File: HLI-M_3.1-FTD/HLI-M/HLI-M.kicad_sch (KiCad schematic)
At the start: 119 parts, among them CON1 , CON2 USB_B, CON3 , CON4 Con_ADAPTER, CON5 Con_MULTLINKER, CON6 Conn_01x15, CON7 Conn_01x09, CON8 CR123A, Q1 DMP3068L-7, Q2 BC817, Q3 BC817, Q4 DMP2305, Q5 DMP2305, Q6 DMP2305, Q7 DMP2305, U1 PIC24HJ64GP206, U10 ULN2003, U11 ULN2003, U12 ULN2003, U2 FM25V10, U3 MAX3232, U4 ATSHA204A-SSHDA-B, U5 24AA02-OT, U6 LM3658SD, U7 TPS7A0533PDBV, U8 TPS7A0533PDBV, U9 FT232RL, Y1 Crystal_32KHz, Y2 Crystal_20MHz

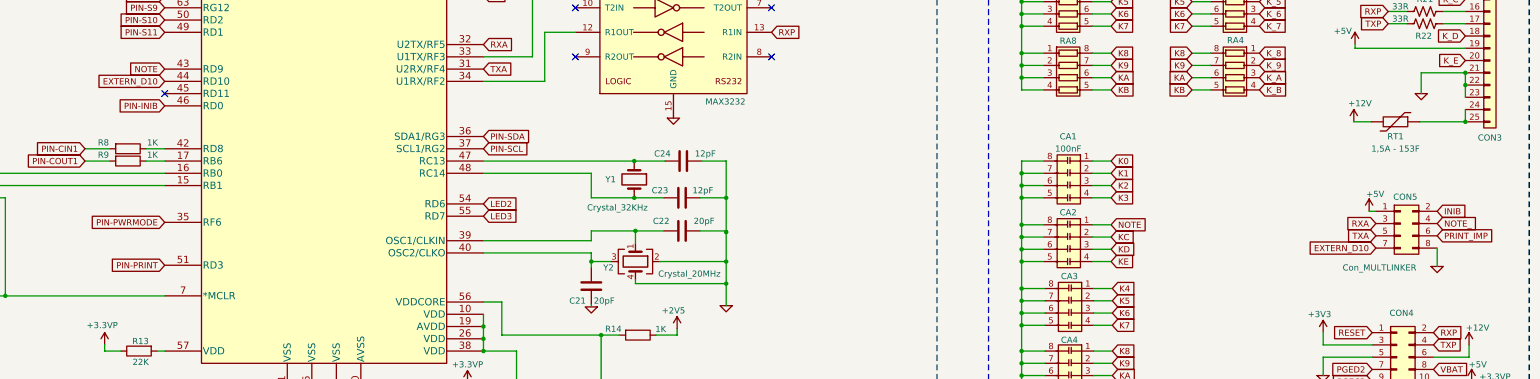
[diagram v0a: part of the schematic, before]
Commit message: att
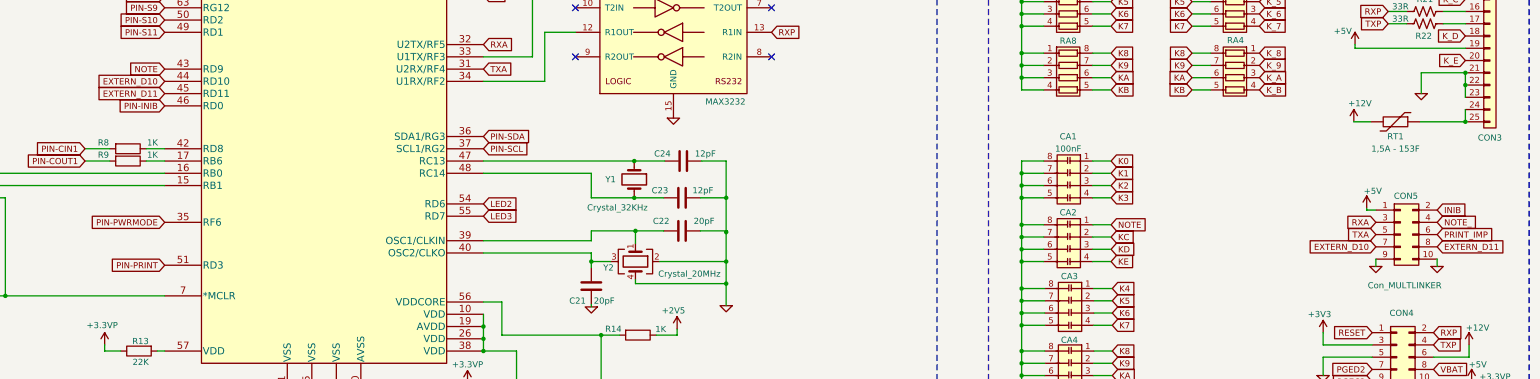
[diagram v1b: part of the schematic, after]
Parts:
- removed CON5: Con_MULTLINKER, Connector_IDC:IDC-Header_2x04_P2.54mm_Horizontal, symbol Connector_Generic:Conn_02x04_Odd_Even
- added CON5: Con_MULTLINKER, Connector_IDC:IDC-Header_2x05_P2.54mm_Horizontal, symbol Connector_Generic:Conn_02x05_Odd_Even
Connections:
- net +5V: now also CON5.1 (Pin_1)
- net 0: now also CON5.10 (Pin_10), CON5.9 (Pin_9)
- net EXTERN_D10: now also CON5.7 (Pin_7)
- net INIB: now also CON5.2 (Pin_2)
- net NOTE_: now also CON5.4 (Pin_4)
- net PRINT_IMP: now also CON5.6 (Pin_6)
- net RXA: now also CON5.3 (Pin_3)
- net TXA: now also CON5.5 (Pin_5)
- net EXTERN_D11: now reaches U1.45 (RD11)
- net EXTERN_D11: now also CON5.8 (Pin_8)
- no-connect marks 35 -> 34
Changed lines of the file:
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@@
   (no_connect (at 77.47 286.258))
   (no_connect (at 132.842 215.392))
-  (no_connect (at 201.168 90.17))
   (no_connect (at 286.258 72.39))
   (no_connect (at 118.11 291.338))
@@
     (stroke (width 0) (type default))
   )
-  (wire (pts (xy 464.82 125.984) (xy 464.82 122.174))
-    (stroke (width 0) (type default))
-  )
   (wire (pts (xy 378.714 117.348) (xy 383.286 117.348))
     (stroke (width 0) (type default))
@@
     (stroke (width 0) (type default))
   )
+  (wire (pts (xy 452.12 125.984) (xy 452.12 124.46))
+    (stroke (width 0) (type default))
+  )
   (wire (pts (xy 392.684 214.122) (xy 392.684 218.186))
     (stroke (width 0) (type default))
@@
     (stroke (width 0) (type default))
   )
+  (wire (pts (xy 464.82 125.984) (xy 464.82 124.46))
+    (stroke (width 0) (type default))
+  )
   (wire (pts (xy 472.44 212.09) (xy 455.422 212.09))
     (stroke (width 0) (type default))
@@
     (stroke (width 0) (type default))
   )
-  (wire (pts (xy 450.723 114.554) (xy 452.12 114.554))
+  (wire (pts (xy 450.215 114.3) (xy 452.12 114.3))
     (stroke (width 0) (type default))
   )
@@
     (stroke (width 0) (type default))
   )
+  (wire (pts (xy 450.215 114.3) (xy 450.215 113.919))
+    (stroke (width 0) (type default))
+  )
   (wire (pts (xy 417.83 68.58) (xy 414.02 68.58))
     (stroke (width 0) (type default))
@@
     )
   )
+  (global_label "EXTERN_D11" (shape input) (at 464.82 121.92 0) (fields_autoplaced)
+    (effects (font (size 1.27 1.27)) (justify left))
+    (property "Intersheetrefs" "${INTERSHEET_REFS}" (at 478.8038 121.92 0)
+      (effects (font (size 1.27 1.27)) (justify left) hide)
+    )
+  )
   (global_label "K6" (shape input) (at 397.256 73.66 0) (fields_autoplaced)
     (effects (font (size 1.27 1.27)) (justify left))
@@
     )
   )
-  (global_label "TXA" (shape input) (at 452.12 119.634 180) (fields_autoplaced)
+  (global_label "TXA" (shape input) (at 452.12 119.38 180) (fields_autoplaced)
     (effects (font (size 1.27 1.27)) (justify right))
-    (property "Intersheetrefs" "${INTERSHEET_REFS}" (at 590.55 476.504 0)
+    (property "Intersheetrefs" "${INTERSHEET_REFS}" (at 590.55 476.25 0)
       (effects (font (size 1.27 1.27)) hide)
     )
@@
     )
   )
-  (global_label "RXA" (shape input) (at 452.12 117.094 180) (fields_autoplaced)
+  (global_label "RXA" (shape input) (at 452.12 116.84 180) (fields_autoplaced)
     (effects (font (size 1.27 1.27)) (justify right))
-    (property "Intersheetrefs" "${INTERSHEET_REFS}" (at 590.55 463.804 0)
+    (property "Intersheetrefs" "${INTERSHEET_REFS}" (at 590.55 463.55 0)
       (effects (font (size 1.27 1.27)) hide)
     )
@@
     )
   )
+  (global_label "EXTERN_D11" (shape input) (at 201.168 90.17 180) (fields_autoplaced)
+    (effects (font (size 1.27 1.27)) (justify right))
+    (property "Intersheetrefs" "${INTERSHEET_REFS}" (at 187.1842 90.17 0)
+      (effects (font (size 1.27 1.27)) (justify right) hide)
+    )
+  )
   (global_label "K6" (shape input) (at 397.51 135.636 0) (fields_autoplaced)
     (effects (font (size 1.27 1.27)) (justify left))
@@
     )
   )
-  (global_label "PRINT_IMP" (shape input) (at 464.82 119.634 0) (fields_autoplaced)
+  (global_label "PRINT_IMP" (shape input) (at 464.82 119.38 0) (fields_autoplaced)
     (effects (font (size 1.27 1.27)) (justify left))
-    (property "Intersheetrefs" "${INTERSHEET_REFS}" (at 996.95 270.764 0)
+    (property "Intersheetrefs" "${INTERSHEET_REFS}" (at 996.95 270.51 0)
       (effects (font (size 1.27 1.27)) hide)
     )
@@
     )
   )
-  (global_label "NOTE_" (shape input) (at 464.82 117.094 0) (fields_autoplaced)
+  (global_label "NOTE_" (shape input) (at 464.82 116.84 0) (fields_autoplaced)
     (effects (font (size 1.27 1.27)) (justify left))
-    (property "Intersheetrefs" "${INTERSHEET_REFS}" (at 1026.16 157.734 0)
+    (property "Intersheetrefs" "${INTERSHEET_REFS}" (at 1026.16 157.48 0)
       (effects (font (size 1.27 1.27)) hide)
     )
@@
     )
   )
-  (global_label "INIB" (shape input) (at 464.82 114.554 0) (fields_autoplaced)
+  (global_label "INIB" (shape input) (at 464.82 114.3 0) (fields_autoplaced)
     (effects (font (size 1.27 1.27)) (justify left))
-    (property "Intersheetrefs" "${INTERSHEET_REFS}" (at 1026.16 180.594 0)
+    (property "Intersheetrefs" "${INTERSHEET_REFS}" (at 1026.16 180.34 0)
       (effects (font (size 1.27 1.27)) hide)
     )
@@
     )
   )
-  (global_label "EXTERN_D10" (shape input) (at 452.12 122.174 180) (fields_autoplaced)
+  (global_label "EXTERN_D10" (shape input) (at 452.12 121.92 180) (fields_autoplaced)
     (effects (font (size 1.27 1.27)) (justify right))
-    (property "Intersheetrefs" "${INTERSHEET_REFS}" (at 438.0634 122.0946 0)
+    (property "Intersheetrefs" "${INTERSHEET_REFS}" (at 438.0634 121.8406 0)
       (effects (font (size 1.27 1.27)) (justify right) hide)
     )
@@
     )
   )
+  (symbol (lib_id "Connector_Generic:Conn_02x05_Odd_Even") (at 457.2 119.38 0) (unit 1)
+    (in_bom yes) (on_board yes) (dnp no)
+    (property "Reference" "CON5" (at 458.343 111.379 0)
+      (effects (font (size 1.27 1.27)))
+    )
+    (property "Value" "Con_MULTLINKER" (at 458.089 129.921 0)
+      (effects (font (size 1.27 1.27)))
+    )
+    (property "Footprint" "Connector_IDC:IDC-Header_2x05_P2.54mm_Horizontal" (at 457.2 119.38 0)
+      (effects (font (size 1.27 1.27)) hide)
+    )
+    (property "Datasheet" "~" (at 457.2 119.38 0)
+      (effects (font (size 1.27 1.27)) hide)
+    )
+    (pin "1")
+    (pin "10")
+    (pin "2")
+    (pin "3")
+    (pin "4")
+    (pin "5")
+    (pin "6")
+    (pin "7")
+    (pin "8")
+    (pin "9")
+    (instances
+      (project "HLI-M"
+        (path "/869d6302-ae22-478f-9723-3feacbb12eef"
+          (reference "CON5") (unit 1)
+        )
+      )
+    )
+  )
   (symbol (lib_id "Device:D") (at 69.2912 234.95 180) (unit 1)
     (in_bom yes) (on_board yes) (dnp no) (fields_autoplaced)
@@
     )
   )
-  (symbol (lib_id "power:+5V") (at 450.723 114.554 0) (unit 1)
+  (symbol (lib_id "power:+5V") (at 450.215 113.919 0) (unit 1)
     (in_bom yes) (on_board yes) (dnp no)
-    (property "Reference" "#PWR0102" (at 450.723 118.364 0)
+    (property "Reference" "#PWR0102" (at 450.215 117.729 0)
       (effects (font (size 1.27 1.27)) hide)
     )
-    (property "Value" "+5V" (at 451.993 110.998 0)
+    (property "Value" "+5V" (at 451.485 110.363 0)
       (effects (font (size 1.27 1.27)))
     )
-    (property "Footprint" "" (at 450.723 114.554 0)
+    (property "Footprint" "" (at 450.215 113.919 0)
       (effects (font (size 1.27 1.27)) hide)
     )
-    (property "Datasheet" "" (at 450.723 114.554 0)
+    (property "Datasheet" "" (at 450.215 113.919 0)
       (effects (font (size 1.27 1.27)) hide)
     )
@@
     )
   )
+  (symbol (lib_id "pspice:0") (at 452.12 125.984 0) (unit 1)
+    (in_bom yes) (on_board yes) (dnp no)
+    (property "Reference" "#GND03" (at 452.12 128.524 0)
+      (effects (font (size 1.27 1.27)) hide)
+    )
+    (property "Value" "0" (at 452.12 123.7234 0)
+      (effects (font (size 1.27 1.27)) hide)
+    )
+    (property "Footprint" "" (at 452.12 125.984 0)
+      (effects (font (size 1.27 1.27)) hide)
+    )
+    (property "Datasheet" "~" (at 452.12 125.984 0)
+      (effects (font (size 1.27 1.27)) hide)
+    )
+    (pin "1")
+    (instances
+      (project "HLI-M"
+        (path "/869d6302-ae22-478f-9723-3feacbb12eef"
+          (reference "#GND03") (unit 1)
+        )
+      )
+    )
+  )
   (symbol (lib_id "pspice:0") (at 464.82 125.984 0) (unit 1)
     (in_bom yes) (on_board yes) (dnp no)
@@
         )
       )
-    )
-  )
-  (symbol (lib_id "Connector_Generic:Conn_02x04_Odd_Even") (at 457.2 117.094 0) (unit 1)
-    (in_bom yes) (on_board yes) (dnp no)
-    (property "Reference" "CON5" (at 458.216 111.5822 0)
-      (effects (font (size 1.27 1.27)))
-    )
-    (property "Value" "Con_MULTLINKER" (at 452.882 126.238 0)
-      (effects (font (size 1.27 1.27)))
-    )
-    (property "Footprint" "Connector_IDC:IDC-Header_2x04_P2.54mm_Horizontal" (at 457.2 117.094 0)
-      (effects (font (size 1.27 1.27)) hide)
-    )
-    (property "Datasheet" "~" (at 457.2 117.094 0)
-      (effects (font (size 1.27 1.27)) hide)
-    )
-    (pin "1")
-    (pin "2")
-    (pin "3")
-    (pin "4")
-    (pin "5")
-    (pin "6")
-    (pin "7")
-    (pin "8")
-    (instances
-      (project "HLI-M"
-        (path "/869d6302-ae22-478f-9723-3feacbb12eef"
-          (reference "CON5") (unit 1)
-        )
-      )
